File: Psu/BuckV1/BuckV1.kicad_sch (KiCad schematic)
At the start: 17 parts, among them J1 IN, J2 OUT, Q1 STD10P6F6, U1 LM2576HVS-ADJ, U2 STPS20M100SG-TR

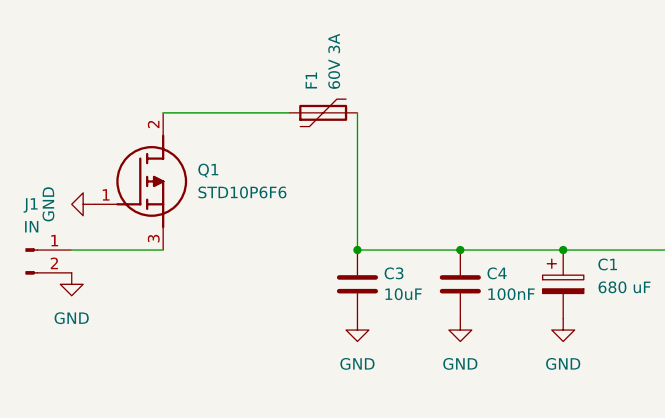
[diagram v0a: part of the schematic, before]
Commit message: raaaa
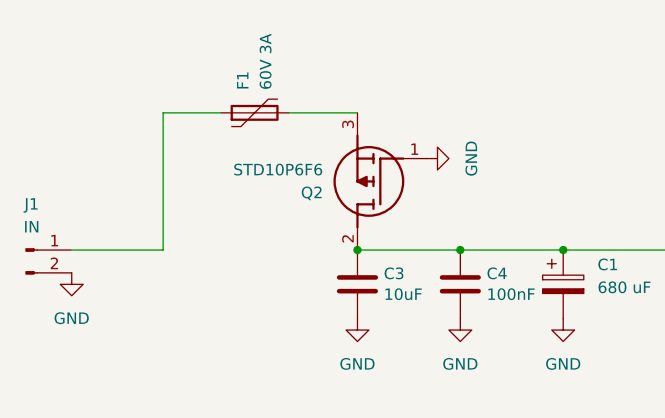
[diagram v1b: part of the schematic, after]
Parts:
- removed Q1: STD10P6F6, STD10P6F6, symbol Personal:STD10P6F6
- added Q2: STD10P6F6, STD10P6F6, symbol Personal:STD10P6F6
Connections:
- net GND: now also Q2.1 (G)
- net at J1.1 (Pin_1): now also F1.1
- net at C1.1, C3.1, C4.1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: now also Q2.2 (D); no longer F1.2
- new net: F1.2, Q2.3 (S)
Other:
- moved on the sheet: F1
